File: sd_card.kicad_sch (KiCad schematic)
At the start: 19 parts, among them U10 TPS22919DCKR, U7 HSP051-4M10, U8 HSP051-4M10, U9 NX3L1T3157GMZ

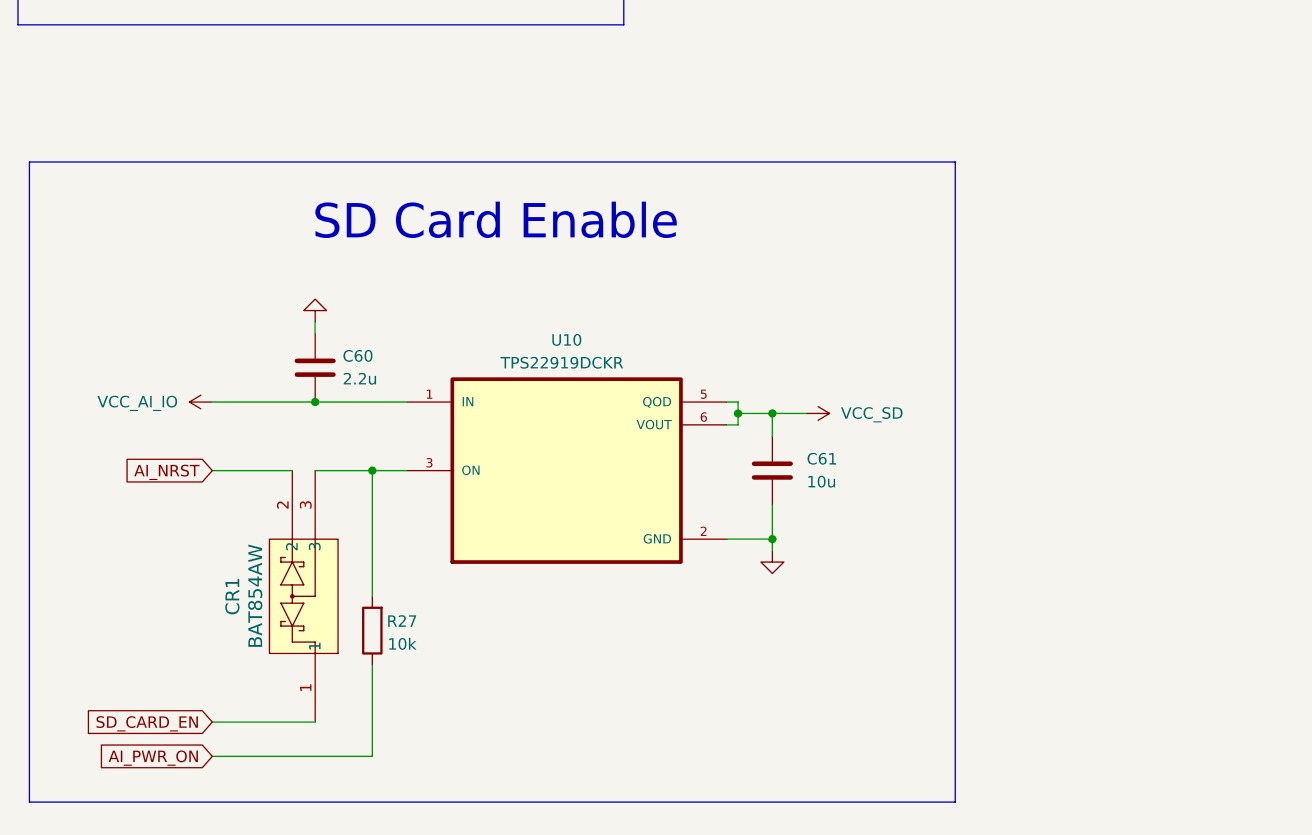
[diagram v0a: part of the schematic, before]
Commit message: Finalize RevB
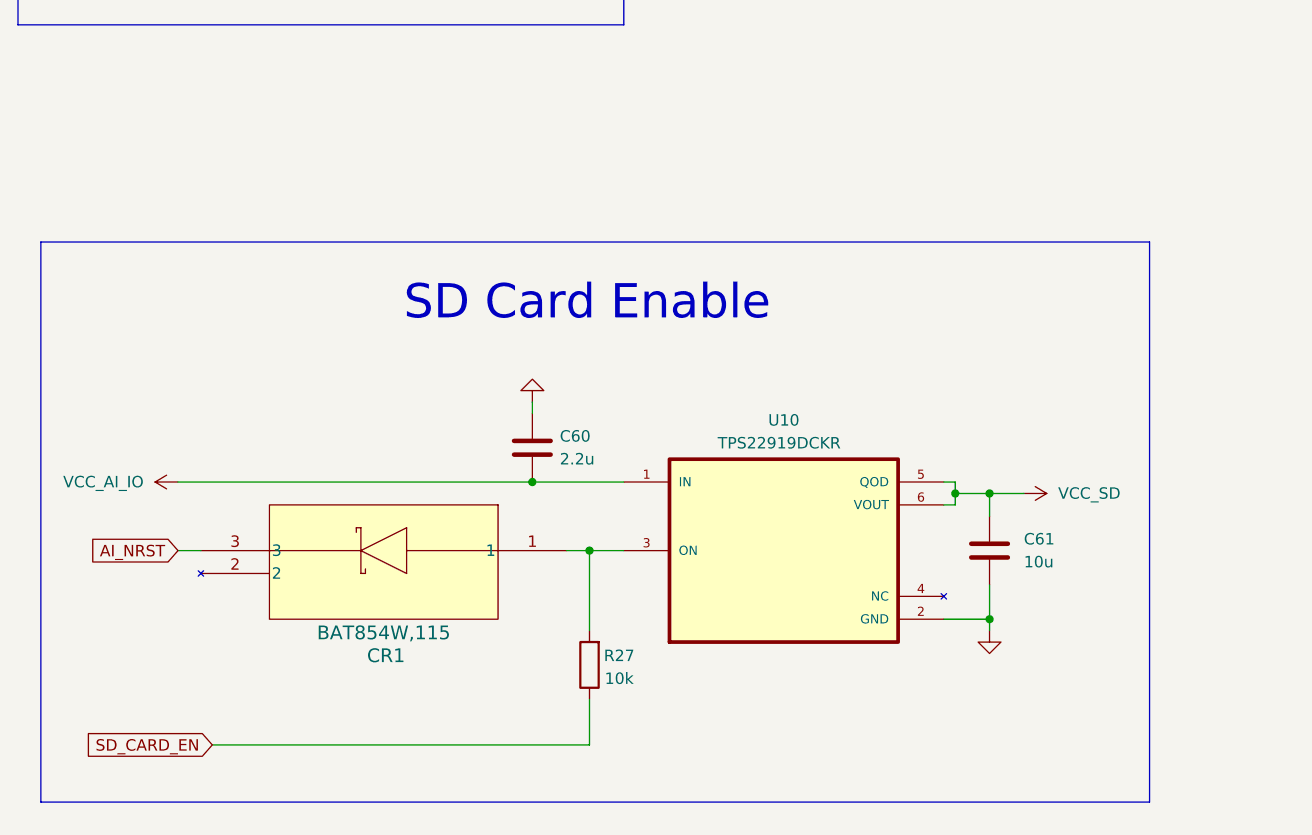
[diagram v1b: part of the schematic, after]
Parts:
- removed CR1: BAT854AW, CivicAlert:BAT854AW,115, symbol BAT854AW,115:BAT854AW
- added CR1: BAT854W,115, CivicAlert:BAT854AW,115, symbol BAT854W,115:BAT854W_115
- C57, C59: MPN (none) -> GRM155R71C104KA88J
- C58, C61: MPN (none) -> GRM188Z71A106KA73D
- C60: MPN (none) -> GRT155C71A225KE13D
- SD1: MPN (none) -> 15882
- U10: MPN (none) -> TPS22919DCKR
- U7, U8: MPN (none) -> HSP051-4M10
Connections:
- net AI_PWR_ON is gone; now on net SD_CARD_EN: R27.1
- net AI_NRST: now also CR1.3
- net at R27.2, U10.3 (ON): now also CR1.1
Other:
- moved on the sheet: C60, C61, R27
